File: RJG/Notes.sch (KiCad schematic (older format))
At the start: 28 parts, among them SW301 Reload, U301 74HCT4051, U302 74HCT40105, U303 74HCT157, U304 74HCT157

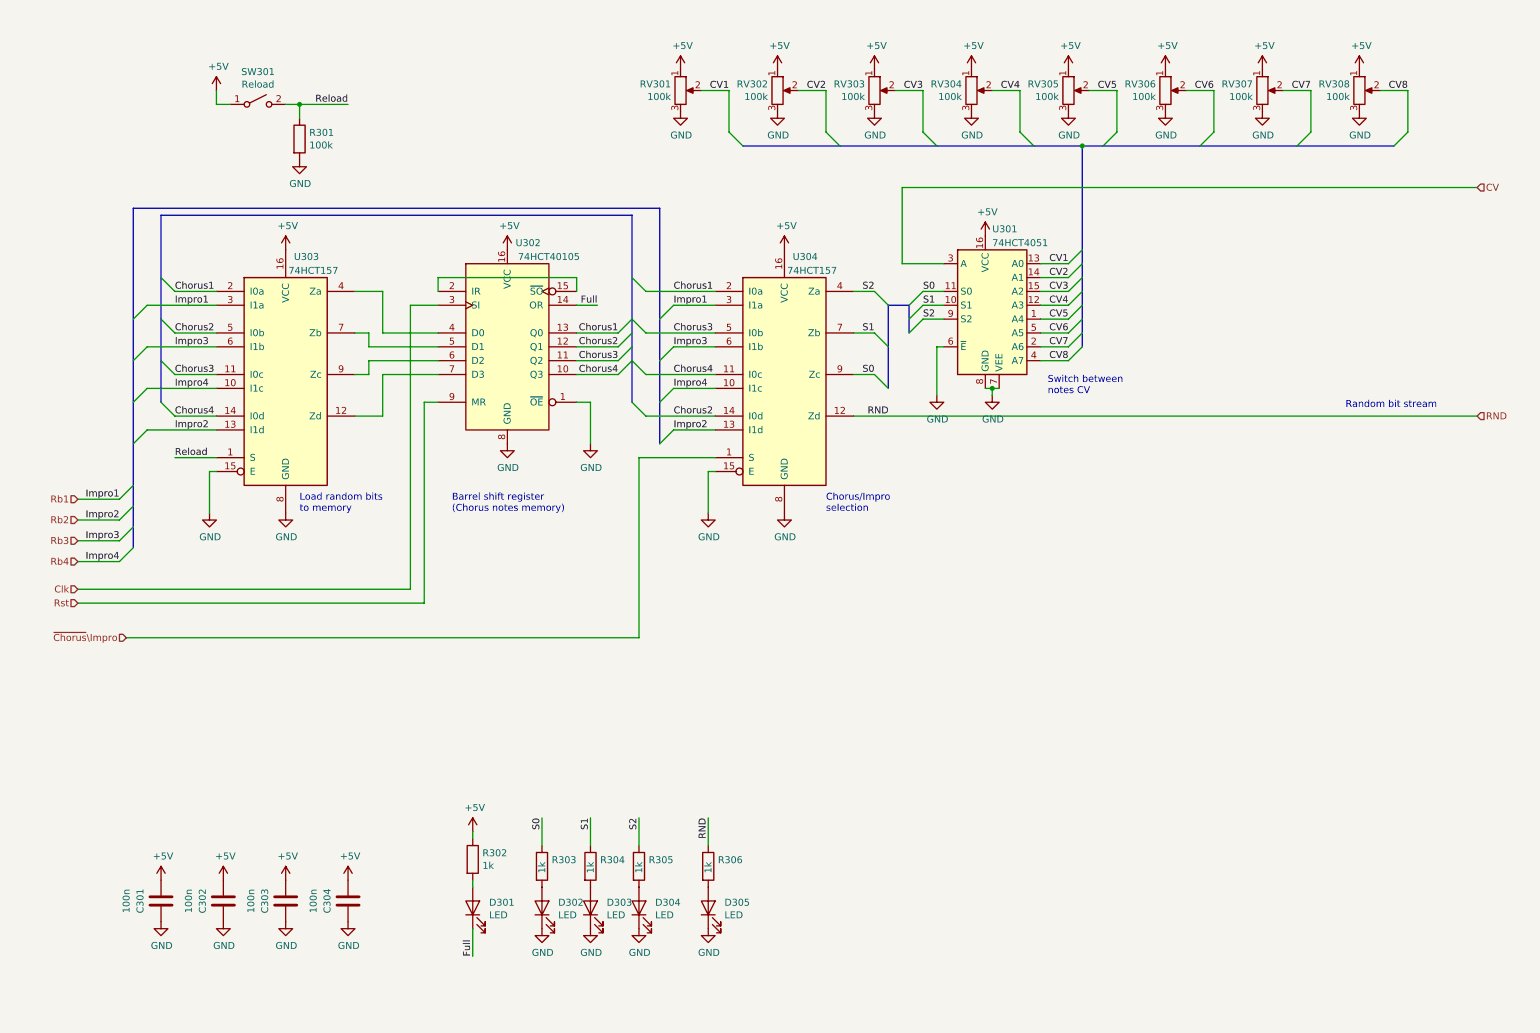
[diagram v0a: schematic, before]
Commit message: fix stuffs
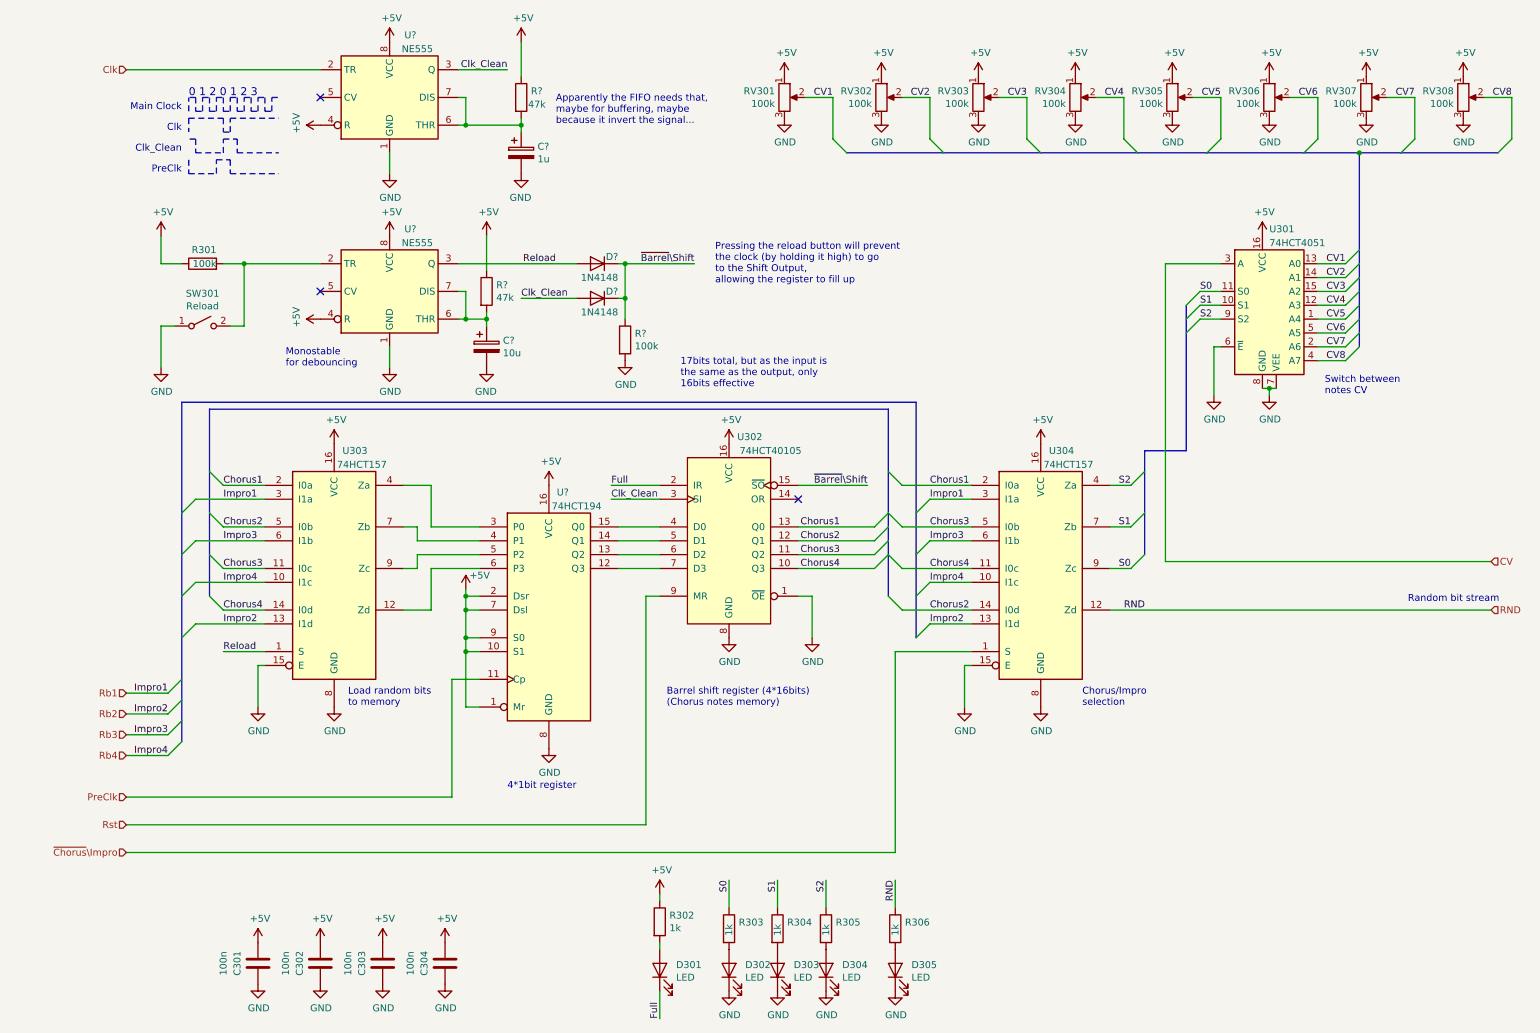
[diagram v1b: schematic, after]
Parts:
- added C?: 1u, Capacitor_THT:CP_Radial_D8.0mm_P3.80mm, symbol Device:CP
- added C?: 10u, Capacitor_THT:CP_Radial_D8.0mm_P3.80mm, symbol Device:CP
- added D? (x2): 1N4148, Diode_THT:D_DO-35_SOD27_P7.62mm_Horizontal, symbol Diode:1N4148
- added R?: 100k, Resistor_THT:R_Axial_DIN0204_L3.6mm_D1.6mm_P7.62mm_Horizontal, symbol Device:R
- added R? (x2): 47k, Resistor_THT:R_Axial_DIN0204_L3.6mm_D1.6mm_P7.62mm_Horizontal, symbol Device:R
- added U?: 74HCT194, symbol 74xx:74LS194
- added U? (x2): NE555, symbol Timer:NE555
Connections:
- net +5V: now also R301.1, R?.1, R?.1, U?.1 (Mr), U?.10 (S1), U?.16 (VCC), U?.2 (Dsr), U?.4 (R), U?.4 (R), U?.7 (Dsl), U?.8 (VCC), U?.8 (VCC), U?.9 (S0); no longer SW301.1 (A)
- net Clk: now also U?.2 (TR); no longer U302.3 (SI)
- net Full: now also U302.2 (IR); no longer U302.14 (OR)
- net GND: now also SW301.1 (A), C?.2, C?.2, R?.2, U?.1 (GND), U?.1 (GND), U?.8 (GND); no longer R301.2
- net Reload: now also D?.2 (A), U?.3 (Q); no longer R301.1, SW301.2 (B)
- net at U303.12 (Zd): now also U?.6 (P3); no longer U302.7 (D3)
- net at U303.4 (Za): now also U?.3 (P0); no longer U302.4 (D0)
- net at U303.7 (Zb): now also U?.4 (P1); no longer U302.5 (D1)
- net at U303.9 (Zc): now also U?.5 (P2); no longer U302.6 (D2)
- net ~Barrel~\Shift: now reaches U302.15 (~SO)
- net ~Barrel~\Shift: now also D?.1 (K), D?.1 (K), R?.1; no longer U302.2 (IR)
- new net: R301.2, SW301.2 (B), U?.2 (TR)
- new net: U302.4 (D0), U?.15 (Q0)
- new net: U302.5 (D1), U?.14 (Q1)
- new net: U302.6 (D2), U?.13 (Q2)
- new net: U302.7 (D3), U?.12 (Q3)
- new net: C?.1, R?.2, U?.6 (THR), U?.7 (DIS) (x2)
- new net Clk_Clean: D?.2 (A), U302.3 (SI), U?.3 (Q)
- new net PreClk: U?.11 (Cp)
- no-connect marks 0 -> 3
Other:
- note added: "0 1 2 0 1 2 3"
- note added: "17bits total, but as the input is\nthe same as the output, only\n16bits effective"
- note added: "4*1bit register"
- note added: "Apparently the FIFO needs that,\nmaybe for buffering, maybe\nbecause it invert the signal..."
- note added: "Barrel shift register (4*16bits)\n(Chorus notes memory)"
- note added: "Clk"
- note added: "Clk_Clean"
- note added: "Main Clock"
- note added: "Monostable \nfor debouncing"
- note added: "PreClk"
- note added: "Pressing the reload button will prevent\nthe clock (by holding it high) to go \nto the Shift Output,\nallowing the register to fill up"
- note removed: "Barrel shift register\n(Chorus notes memory)"
- moved on the sheet: C301, C302, C303, C304, D301, D302, D303, D304, D305, R301, R302, R303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
